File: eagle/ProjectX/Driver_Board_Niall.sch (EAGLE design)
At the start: 188 parts, among them IC2 NCV78M05BDTRKG, J1 694102303002, U1 TC4427AEOA, U10 TC4427AEOA, U11 TC4427AEOA, U12 TC4427AEOA, U1200 CD74HC4067SM96, U13 TC4427AEOA, U14 TC4427AEOA, U15 TC4427AEOA, U16 TC4427AEOA, U17 TC4427AEOA, U18 TC4427AEOA, U19 TC4427AEOA, U2 TC4427AEOA, U20 TC4427AEOA, U200 ADA4091-2ARZ-RL, U21 TC4427AEOA, U22 TC4427AEOA, U23 TC4427AEOA, U24 TC4427AEOA, U25 TC4427AEOA, U26 TC4427AEOA, U27 TC4427AEOA, U28 TC4427AEOA, U29 TC4427AEOA, U3 TC4427AEOA, U30 TC4427AEOA, U31 TC4427AEOA, U32 TC4427AEOA, U33 TC4427AEOA, U34 TC4427AEOA, U35 TC4427AEOA, U36 TC4427AEOA, U37 TC4427AEOA, U38 TC4427AEOA, U39 TC4427AEOA, U4 TC4427AEOA, U40 TC4427AEOA, U41 TC4427AEOA, U42 TC4427AEOA, U43 TC4427AEOA, U44 TC4427AEOA, U45 TC4427AEOA, U46 TC4427AEOA, U47 TC4427AEOA, U48 TC4427AEOA, U49 TC4427AEOA, U5 TC4427AEOA, U50 TC4427AEOA, U6 TC4427AEOA, U7 TC4427AEOA, U8 TC4427AEOA, U9 TC4427AEOA

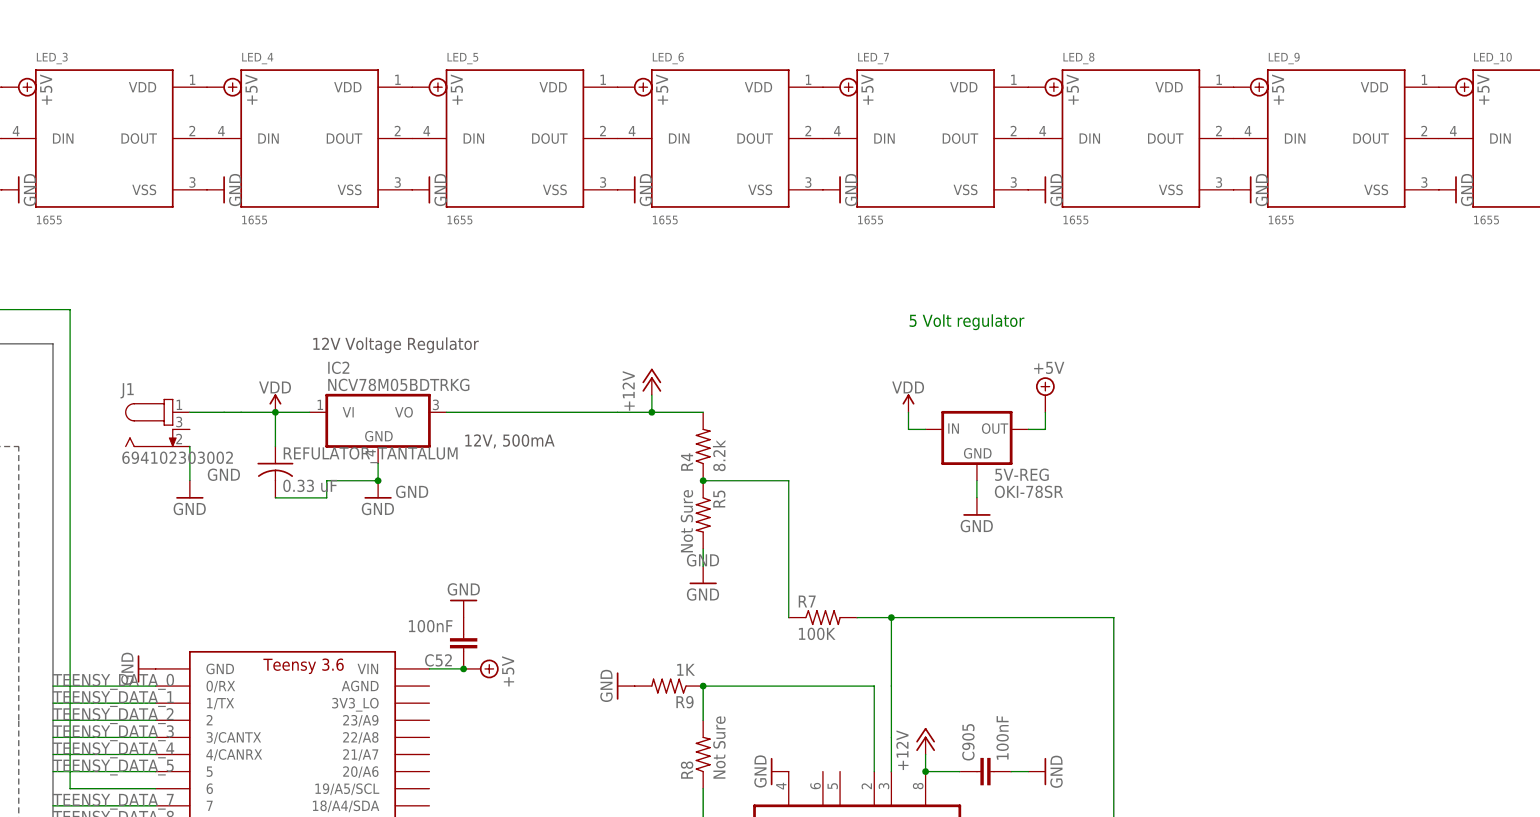
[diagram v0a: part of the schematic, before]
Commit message: Bit more work
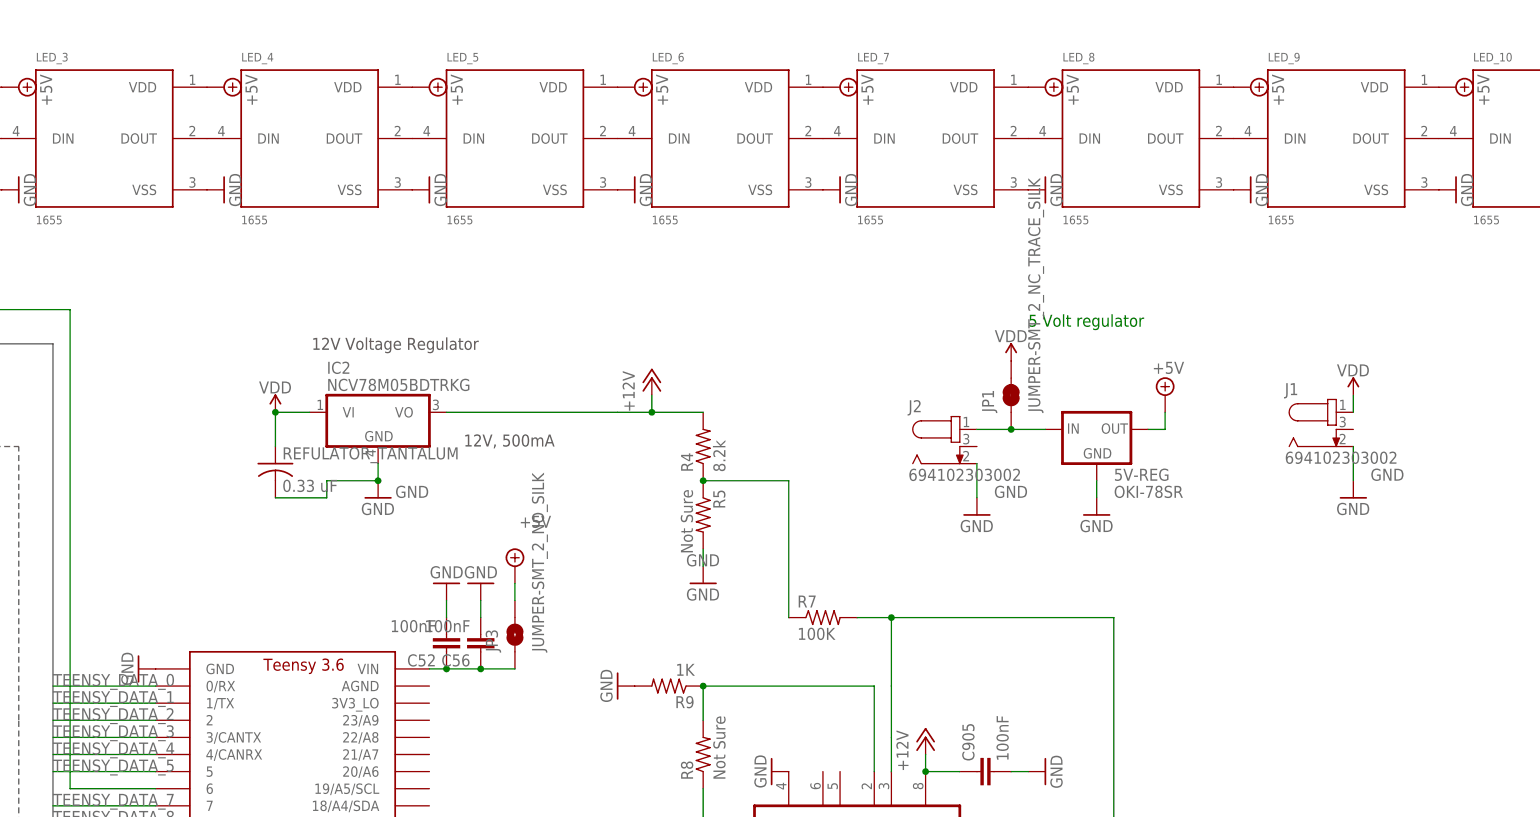
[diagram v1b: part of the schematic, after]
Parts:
- added C56: 100nF, resistor:C-EUC0805
- added J2: 694102303002, SnapEDA-Library:694102303002
- added JP1: JUMPER-SMT_2_NC_TRACE_SILK, SparkFun-Jumpers:JUMPER-SMT_2_NC_TRACE_SILK
- added JP3: JUMPER-SMT_2_NO_SILK, SparkFun-Jumpers:JUMPER-SMT_2_NO_SILK
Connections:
- new net N$24: 5V-REG.IN, J2.1, JP1.1
- new net N$25: C52.1, C56.1, JP3.1, U$1.VIN
- net +5V: now also JP3.2; no longer C52.1, U$1.VIN
- net GND: now also C56.2, J2.2
- net VDD: now also JP1.2; no longer 5V-REG.IN
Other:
- moved on the sheet: 5V-REG, C52, J1
